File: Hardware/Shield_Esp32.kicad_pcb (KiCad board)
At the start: 2 copper layers, 81.9 x 53.8 mm, 43 parts, among them J1 Conn_01x02_Male, J10 Conn_01x02_Male, J11 Conn_01x02_Male, J12 Conn_01x02_Male, J13 Conn_01x02_Male, J14 Conn_01x02_Male, J15 Conn_01x02_Male, J16 Conn_01x02_Male, J17 Conn_01x02_Male, J18 Conn_01x02_Male, J19 Conn_01x02_Male, J2 Conn_01x02_Male, J20 Conn_01x02_Male, J21 Conn_01x02_Male, J22 Conn_01x02_Male, J23 Conn_01x02_Male, J3 Conn_02x13_Odd_Even, J4 Conn_01x15, J5 Conn_01x15, J6 Conn_01x02_Male, J7 Conn_01x02_Male, J8 Conn_01x03_Male, J9 Conn_01x02_Male

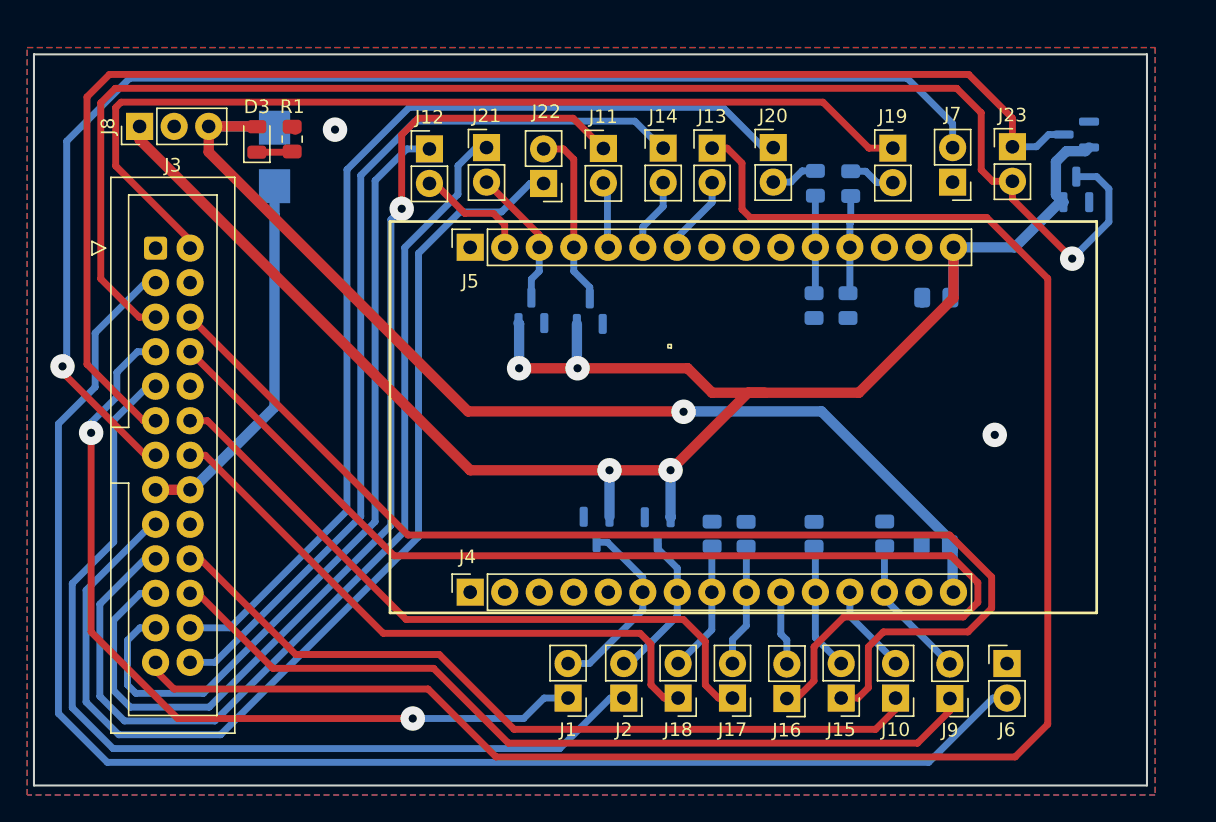
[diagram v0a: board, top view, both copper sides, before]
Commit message: pcb update + new pcb
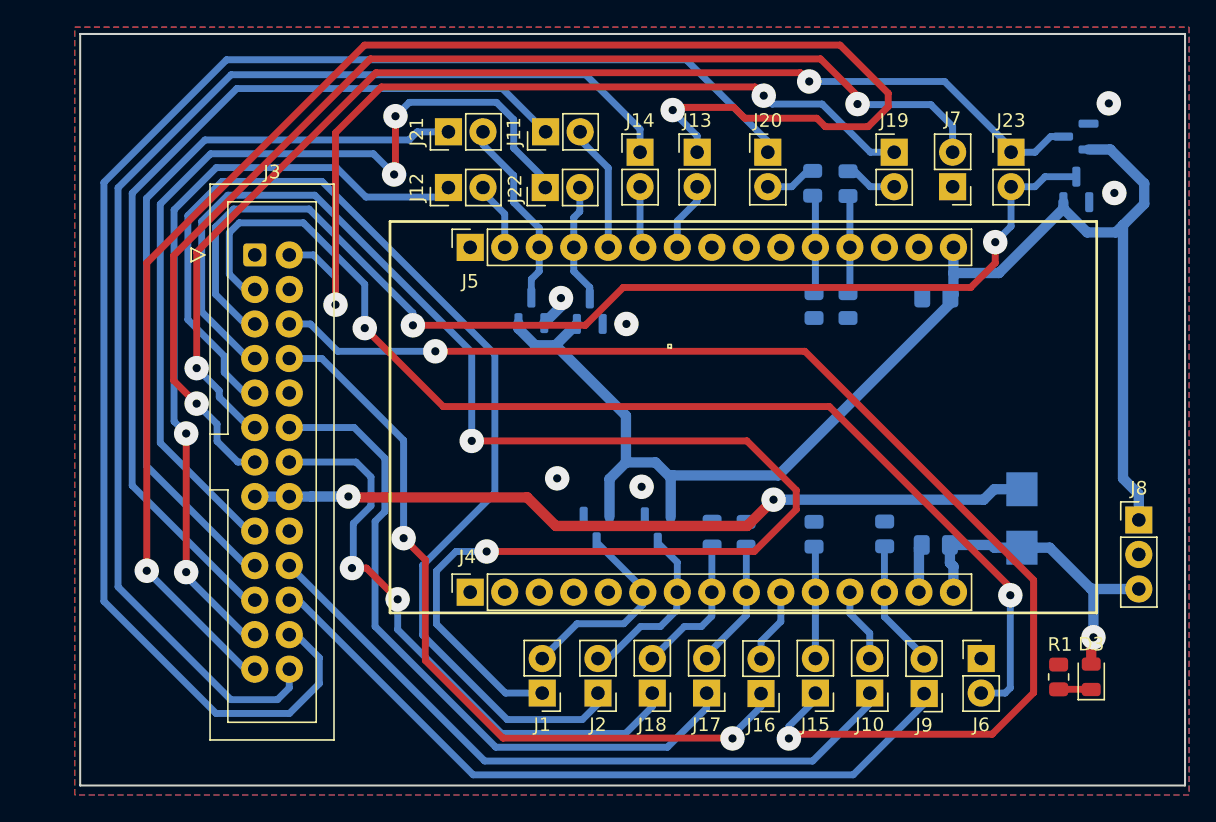
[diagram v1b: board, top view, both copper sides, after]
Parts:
- moved J8 79.0 mm to (202.8, 107.8), turned to 0 degrees
- moved D3 73.0 mm to (199.3, 119.3)
- moved R1 68.9 mm to (196.9, 119.3)
- moved D4 61.1 mm to (194.2, 107.7), turned to 90 degrees
- moved J3 7.32 mm to (137.7, 88.3)
- moved J11 4.42 mm to (159.2, 79.2), turned to 90 degrees
- moved J12 3.17 mm to (152.0, 83.3), turned to 90 degrees
- moved J21 3.03 mm to (152.0, 79.2), turned to 90 degrees
- moved J16 1.93 mm to (175.0, 120.5)
- moved J6 1.93 mm to (191.2, 118.0)
- moved J9 1.93 mm to (187.0, 120.5)
- moved J1 1.93 mm to (158.9, 120.5)
- moved J10 1.93 mm to (183.0, 120.5)
- moved J15 1.93 mm to (179.0, 120.5)
- moved J17 1.93 mm to (171.0, 120.5)
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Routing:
- net +5V: track 80.7 -> 24.4 mm
- net ADC0: track 61.7 -> 112.9 mm
- net ENC1: track 74.7 -> 111.7 mm
- net +5VP: track 27.5 -> 58.5 mm, vias 0 -> 2
- net TRIG1: track 84.9 -> 56.9 mm, vias 0 -> 2
- net +3.3V: track 131.6 -> 104.8 mm, vias 4 -> 0
- net PWM2N: track 66.8 -> 92.4 mm
- net ADC3: track 107.5 -> 83.9 mm, vias 1 -> 2
- net AMP1: track 108.4 -> 85.9 mm, vias 0 -> 2
- net RXB: track 72.4 -> 54.9 mm
- net ADC2: track 102.8 -> 87.3 mm, vias 0 -> 2
- net PWM2: track 133.4 -> 118.2 mm, vias 0 -> 2
- net ADC1: track 69.9 -> 84.0 mm
- net TXB: track 79.0 -> 66.5 mm, vias 0 -> 2
- net PWM1: track 80.9 -> 69.0 mm, vias 1 -> 0
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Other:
- board size 81.9 x 53.8 mm -> 81.3 x 55.3 mm
